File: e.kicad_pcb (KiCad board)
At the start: 2 copper layers, 78 x 58.3 mm, 9 parts, among them SW1 usr, SW2 rst, U1 Display_ST7789, U2 MAX98357A

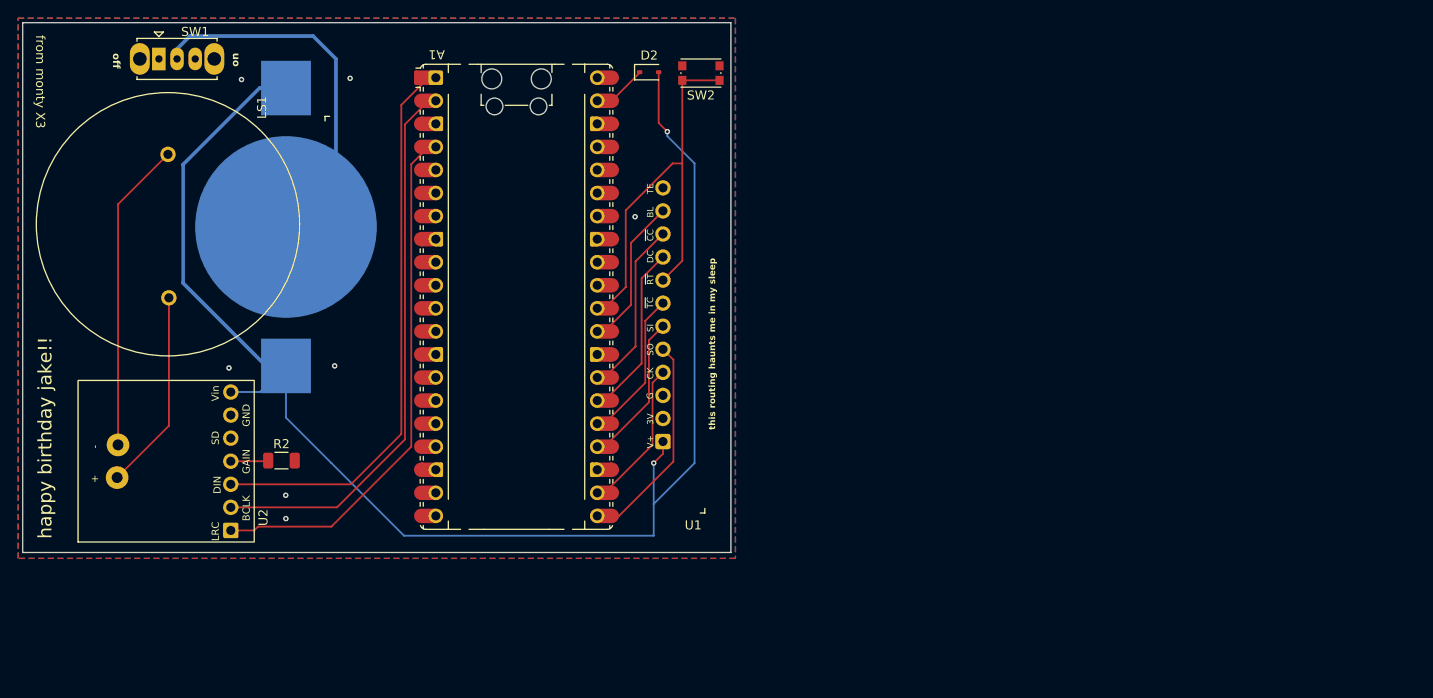
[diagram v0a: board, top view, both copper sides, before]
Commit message: pcb layout done!!
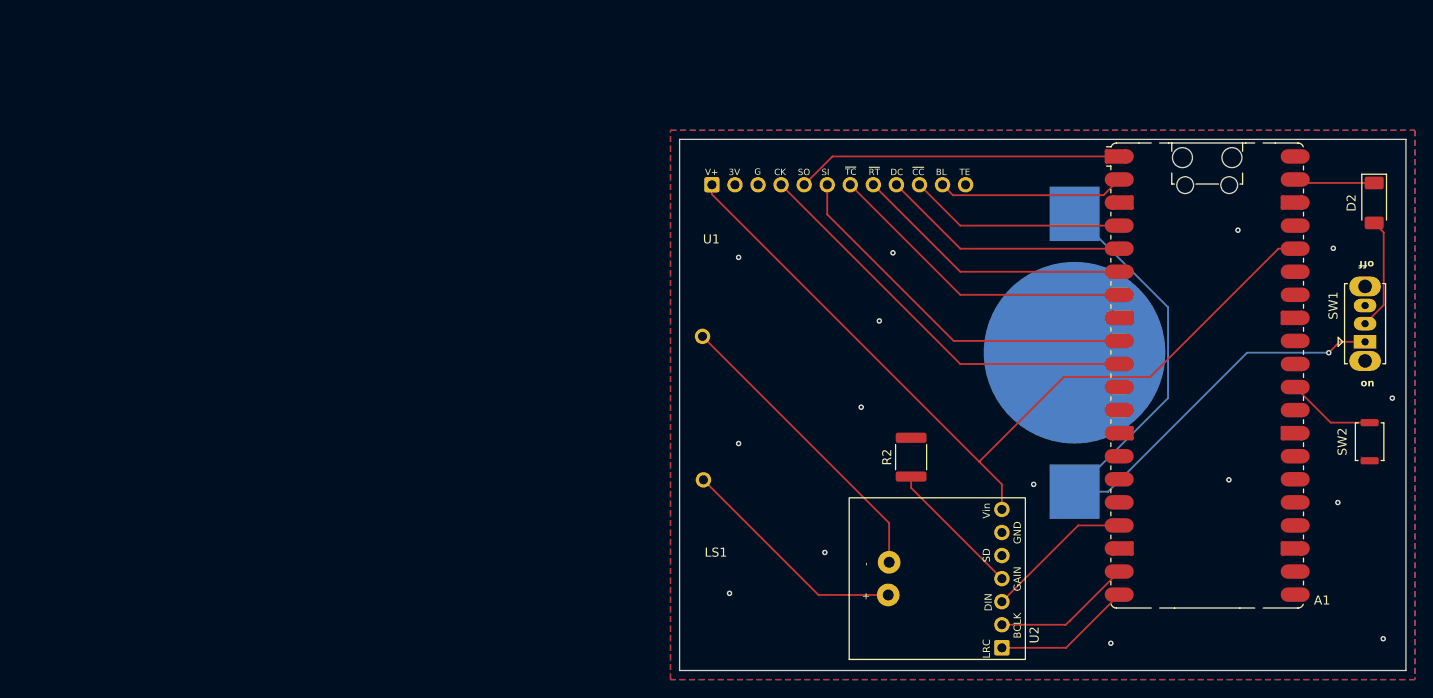
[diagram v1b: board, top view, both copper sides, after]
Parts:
- A1: footprint Module:RaspberryPi_Pico_Common_Unspecified -> Module:RaspberryPi_Pico_Common_SMD
- BT1: value CR2430 -> CR2450
- D2: footprint Diode_SMD:D_SOD-323 -> Diode_SMD:D_SOD-128
- R2: footprint Resistor_SMD:R_1206_3216Metric -> Resistor_SMD:R_1812_4532Metric
- SW2: footprint Button_Switch_SMD:SW_Push_1P1T_NO_CK_KMR2 -> Button_Switch_SMD:SW_Push_SPST_NO_Alps_SKRK
- moved SW1 136.5 mm to (260.0, 101.3), turned to 90 degrees
- moved BT1 87.9 mm to (228.0, 102.5), turned to 90 degrees
- moved U2 85.9 mm to (213.1, 127.4)
- moved SW2 84.1 mm to (260.5, 112.3), turned to 90 degrees
- moved D2 81.1 mm to (261.0, 86.0), turned to -90 degrees
- moved A1 76.6 mm to (242.6, 105.0)
- moved R2 69.4 mm to (210.0, 114.0), turned to 90 degrees
- moved LS1 62.2 mm to (186.5, 108.4)
- moved U1 46.9 mm to (202.0, 67.8), turned to 0 degrees
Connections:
- A1 pad 10: unconnected-(A1-GPIO7-Pad10) -> Net-(A1-GPIO7)
- A1 pad 17: unconnected-(A1-GPIO13-Pad17) -> Net-(A1-GPIO13)
- A1 pad 19: unconnected-(A1-GPIO14-Pad19)_1 -> Net-(A1-GPIO14)
- A1 pad 20: unconnected-(A1-GPIO15-Pad20)_1 -> Net-(A1-GPIO15)
- A1 pad 21: Net-(A1-GPIO16) -> unconnected-(A1-GPIO16-Pad21)
- A1 pad 22: Net-(A1-GPIO17) -> unconnected-(A1-GPIO17-Pad22)
- A1 pad 24: Net-(A1-GPIO18) -> unconnected-(A1-GPIO18-Pad24)
- A1 pad 25: Net-(A1-GPIO19) -> unconnected-(A1-GPIO19-Pad25)
- A1 pad 26: Net-(A1-GPIO20) -> unconnected-(A1-GPIO20-Pad26)
- A1 pad 27: Net-(A1-GPIO21) -> unconnected-(A1-GPIO21-Pad27)
- A1 pad 29: Net-(A1-GPIO22) -> unconnected-(A1-GPIO22-Pad29)
- A1 pad 33: unconnected-(A1-AGND-Pad33) -> GND
- A1 pad 36: unconnected-(A1-3V3-Pad36)_1 -> PICO_PWR
- A1 pad 5: unconnected-(A1-GPIO3-Pad5) -> Net-(A1-GPIO3)
- A1 pad 6: unconnected-(A1-GPIO4-Pad6) -> Net-(A1-GPIO4)
- A1 pad 7: unconnected-(A1-GPIO5-Pad7) -> Net-(A1-GPIO5)
- A1 pad 9: unconnected-(A1-GPIO6-Pad9)_1 -> Net-(A1-GPIO6)
- BT1 pad 1: +3V0 -> Net-(BT1-+)
- BT1 pad 2: Net-(BT1--) -> GND
- SW1 pad 1: GND -> Net-(BT1-+)
- SW1 pad 2: Net-(BT1--) -> +3V0
- SW2 pad 1: Net-(A1-RUN) -> GND
- SW2 pad 2: GND -> Net-(A1-RUN)
- U1 pad 1: +3V0 -> PICO_PWR
- U1 pad 10: Net-(A1-GPIO21) -> Net-(A1-GPIO2)
- U1 pad 11: Net-(A1-GPIO22) -> Net-(A1-GPIO1)
- U1 pad 4: Net-(A1-GPIO17) -> Net-(A1-GPIO7)
- U1 pad 5: Net-(A1-GPIO16) -> Net-(A1-GPIO0)
- U1 pad 6: Net-(A1-GPIO18) -> Net-(A1-GPIO6)
- U1 pad 7: Net-(A1-GPIO19) -> Net-(A1-GPIO5)
- U1 pad 8: Net-(A1-RUN) -> Net-(A1-GPIO4)
- U1 pad 9: Net-(A1-GPIO20) -> Net-(A1-GPIO3)
- U2 pad 1: Net-(A1-GPIO2) -> Net-(A1-GPIO15)
- U2 pad 2: Net-(A1-GPIO1) -> Net-(A1-GPIO14)
- U2 pad 3: Net-(A1-GPIO0) -> Net-(A1-GPIO13)
- U2 pad 7: +3V0 -> PICO_PWR
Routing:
- net +3V0: track 163.7 -> 12.4 mm, vias 2 -> 0
- net PICO_PWR: track 0.00 -> 93.5 mm
- net Net-(BT1-+): track 0.00 -> 78.0 mm, vias 0 -> 1
- net Net-(A1-GPIO7): track 0.00 -> 45.4 mm
- net Net-(BT1--): track 44.6 -> 0.00 mm
- net Net-(A1-GPIO6): track 0.00 -> 41.2 mm
- net Net-(A1-GPIO1): track 60.7 -> 20.7 mm
- net Net-(A1-RUN): track 47.1 -> 9.82 mm
- net Net-(A1-GPIO5): track 0.00 -> 34.6 mm
- net Net-(A1-GPIO2): track 57.5 -> 23.9 mm
- net Net-(A1-GPIO4): track 0.00 -> 31.0 mm
- net Net-(A1-GPIO3): track 0.00 -> 27.5 mm
- net Net-(A1-GPIO0): track 61.6 -> 36.0 mm
- net Net-(A1-GPIO16): track 22.9 -> 0.00 mm
- net Net-(A1-GPIO21): track 18.5 -> 0.00 mm
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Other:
- board size 78 x 58.3 mm -> 80 x 58.5 mm
- board text removed: "from monty X3"
- board text removed: "happy birthday jake!!"
- board text removed: "this routing haunts me in my sleep"
